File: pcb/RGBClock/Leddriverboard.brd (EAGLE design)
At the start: 100 x 80 mm, 37 parts, among them U1 LP3878MR-ADJ, U2 P82B96DR, U3 PCA9685PW, U4 ZXLD1362ET5TA, U5 ZXLD1362ET5TA, U6 ZXLD1362ET5TA, X2 43045-0600, X3 43045-0400

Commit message: Cleanup schematic
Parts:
- renumbered X3 to X1
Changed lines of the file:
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@@
 <element name="R6" library="resistor" package="R0402" value="A1-0" x="35.56" y="12.7"/>
 <element name="R4" library="resistor" package="R0402" value="A2-0" x="35.56" y="11.43"/>
-<element name="X3" library="con-molex-micro-fit-3_0" package="43045-0400" value="43045-0400" x="5.08" y="6.35" rot="R270">
+<element name="X1" library="con-molex-micro-fit-3_0" package="43045-0400" value="43045-0400" x="5.08" y="6.35" rot="R270">
 <attribute name="MATERIAL" value="" x="5.08" y="6.35" size="1.778" layer="27" rot="R270" display="off"/>
 </element>
@@
 <contactref element="R9" pad="1"/>
 <contactref element="R6" pad="1"/>
-<contactref element="X3" pad="P$1"/>
+<contactref element="X1" pad="P$1"/>
 <wire x1="55.88" y1="28.3972" x2="62.1284" y2="29.21" width="0" layer="19" extent="1-1"/>
 <wire x1="62.1284" y1="17.78" x2="62.1284" y2="29.21" width="0" layer="19" extent="1-1"/>
@@
 <contactref element="U2" pad="6"/>
 <contactref element="D2" pad="KAT"/>
-<contactref element="X3" pad="P$2"/>
+<contactref element="X1" pad="P$2"/>
 <wire x1="27.8638" y1="6.985" x2="27.8638" y2="5.715" width="0" layer="19" extent="1-1"/>
 <wire x1="17.83" y1="1.6" x2="27.8638" y2="5.715" width="0" layer="19" extent="1-1"/>
@@
 <contactref element="U2" pad="2"/>
 <contactref element="D3" pad="KAT"/>
-<contactref element="X3" pad="P$3"/>
+<contactref element="X1" pad="P$3"/>
 <wire x1="22.9362" y1="6.985" x2="22.9362" y2="8.255" width="0" layer="19" extent="1-1"/>
 <wire x1="17.73" y1="12.37" x2="22.9362" y2="8.255" width="0" layer="19" extent="1-1"/>
@@
 <signal name="N$25">
 <contactref element="D1" pad="A"/>
-<contactref element="X3" pad="P$4"/>
+<contactref element="X1" pad="P$4"/>
 <wire x1="12.4" y1="7.85" x2="13.97" y2="3.81" width="0" layer="19" extent="1-1"/>
 </signal>

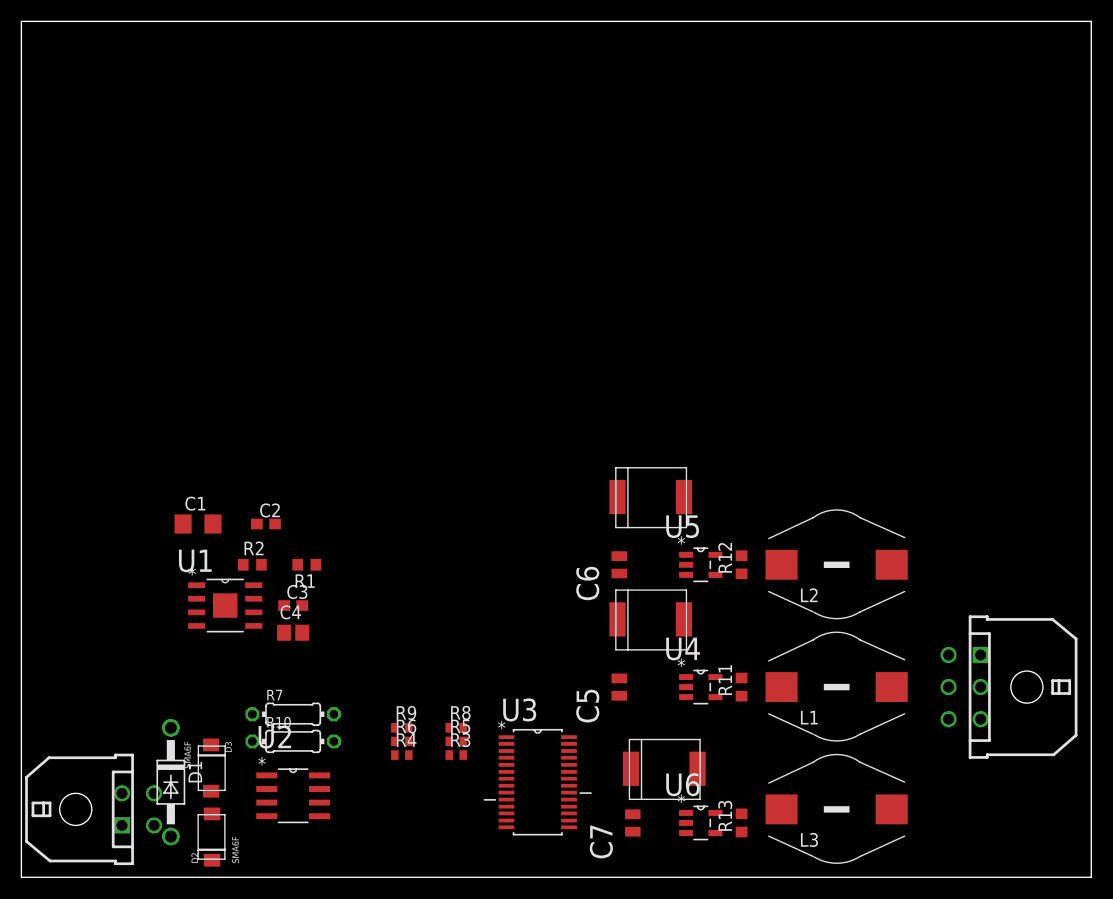
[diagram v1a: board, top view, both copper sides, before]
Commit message: Led driver
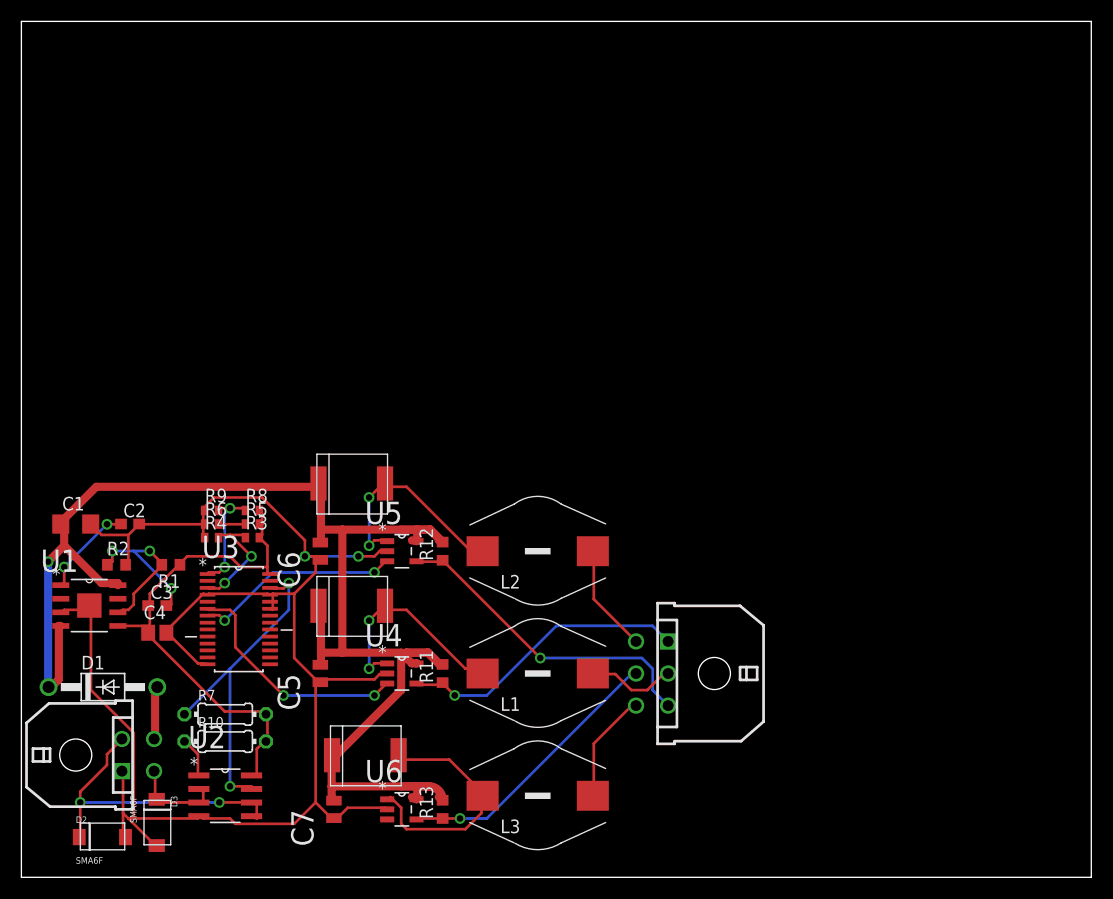
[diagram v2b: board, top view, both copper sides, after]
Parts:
- moved U3 31.8 mm to (20.3, 24.1)
- moved X2 29.2 mm to (64.8, 19.1)
- moved L1 28.0 mm to (48.3, 19.1)
- moved L2 28.0 mm to (48.3, 30.5)
- moved L3 28.0 mm to (48.3, 7.62)
- moved R11 28.0 mm to (39.4, 19.1)
- moved R12 28.0 mm to (39.4, 30.5)
- moved R13 28.0 mm to (39.4, 6.35)
- moved C5 28.0 mm to (27.9, 19.1)
- moved C6 28.0 mm to (27.9, 30.5)
- moved D6 28.0 mm to (30.5, 11.4)
- moved C7 28.0 mm to (29.2, 6.35)
- moved D4 28.0 mm to (29.2, 25.4)
- moved D5 28.0 mm to (29.2, 36.8)
- moved U4 28.0 mm to (35.6, 19.1)
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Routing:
- net GND: track 0.00 -> 153.7 mm, vias 0 -> 2
- net VCC: track 0.00 -> 135.1 mm, vias 0 -> 1
- net +5V: track 0.00 -> 48.1 mm
- net SCL: track 0.00 -> 31.5 mm, vias 0 -> 2
- net N$4: track 0.00 -> 30.3 mm, vias 0 -> 1
- net N$22: track 0.00 -> 29.3 mm, vias 0 -> 2
- net N$1: track 0.00 -> 27.4 mm, vias 0 -> 1
- net N$16: track 0.00 -> 26.2 mm, vias 0 -> 1
- net N$19: track 0.00 -> 22.9 mm
- net N$8: track 0.00 -> 22.3 mm, vias 0 -> 2
- net N$10: track 0.00 -> 20.6 mm, vias 0 -> 2
- net N$9: track 0.00 -> 20.3 mm, vias 0 -> 2
- net N$24: track 0.00 -> 20.2 mm, vias 0 -> 3
- net N$2: track 0.00 -> 19.3 mm, vias 0 -> 2
- net N$43: track 0.00 -> 11.2 mm, vias 0 -> 2
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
